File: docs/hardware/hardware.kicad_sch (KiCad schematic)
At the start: 8 parts, among them J1 BASYS_JA, J2 AudioJack2, J6 BASYS_JB, J7 GAMEPAD_1, J8 GAMEPAD_2

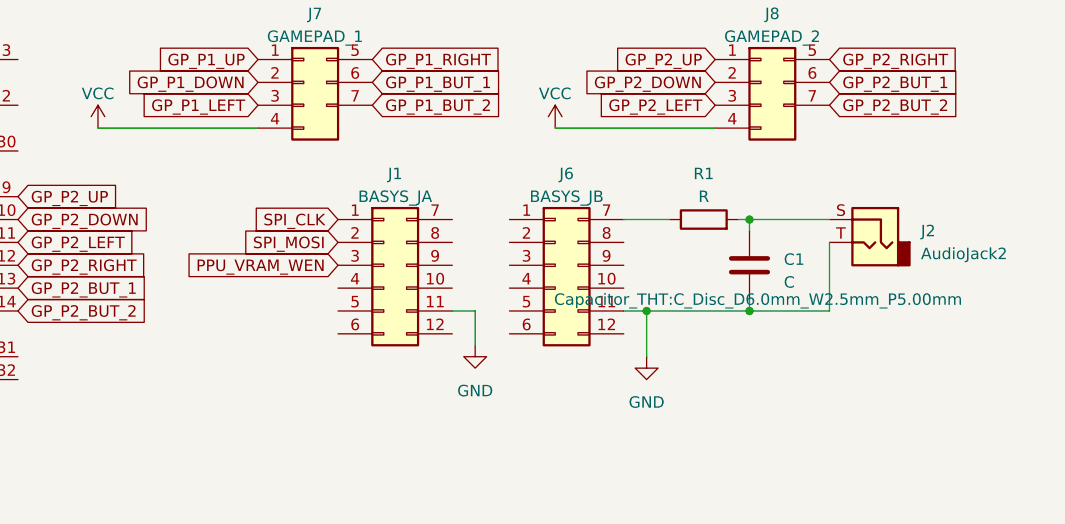
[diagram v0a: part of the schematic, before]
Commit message: WIP ppu testing
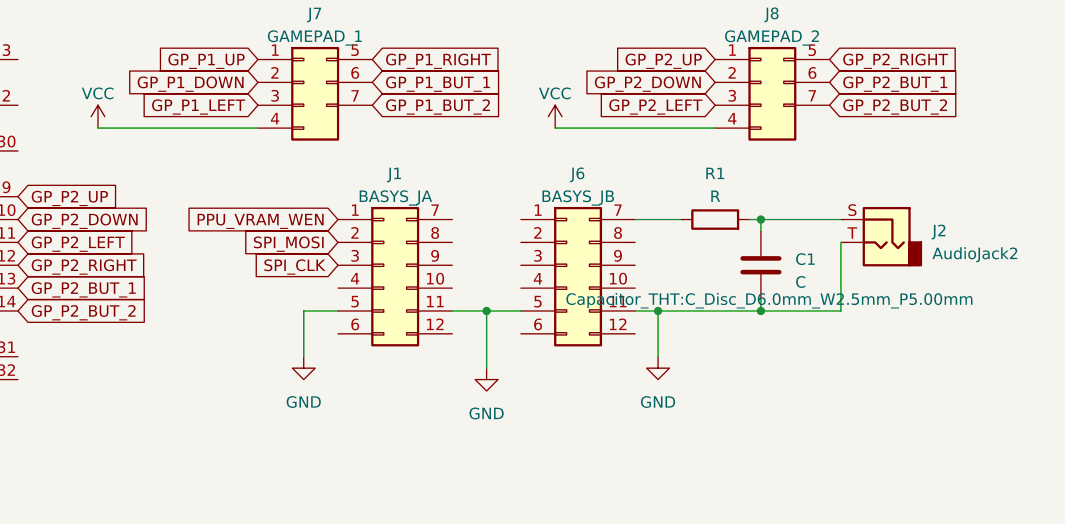
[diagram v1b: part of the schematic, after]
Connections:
- net GND: now also J1.5 (Pin_5), J6.5 (Pin_5)
- net PPU_VRAM_WEN: now also J1.1 (Pin_1); no longer J1.3 (Pin_3)
- net SPI_CLK: now also J1.3 (Pin_3); no longer J1.1 (Pin_1)
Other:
- moved on the sheet: C1, J2, J6, R1

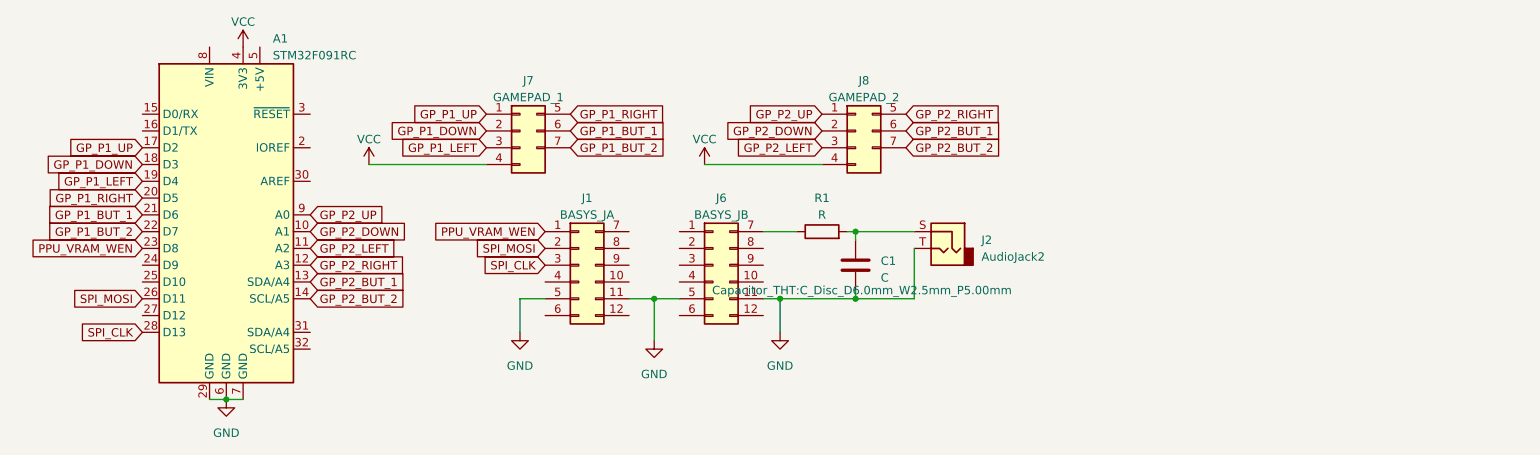
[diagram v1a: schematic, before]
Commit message: finalize hardware
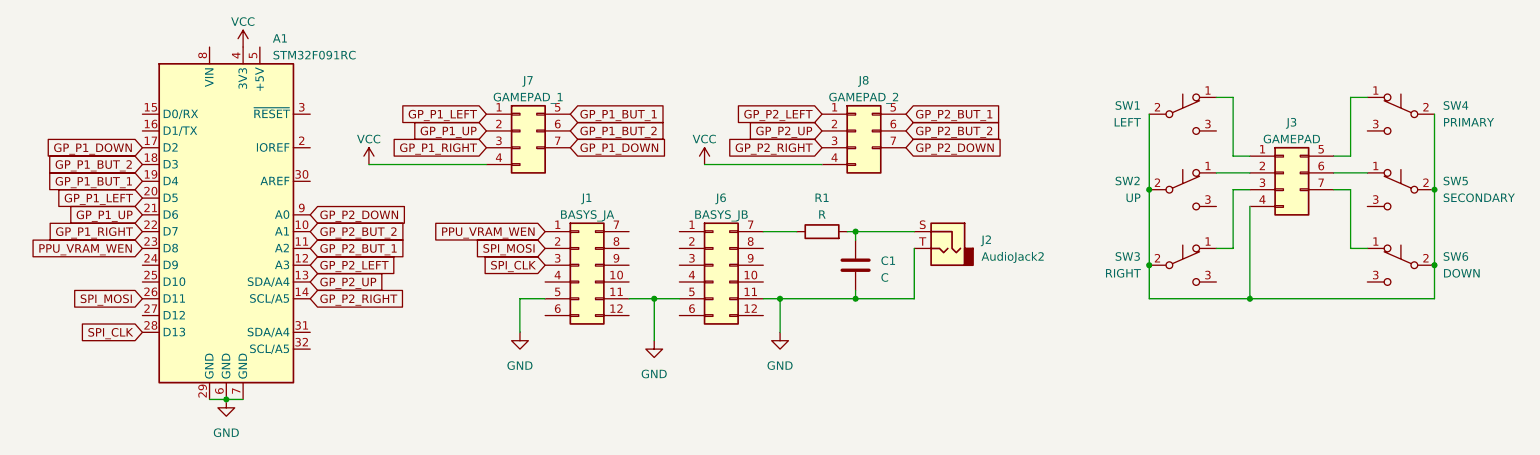
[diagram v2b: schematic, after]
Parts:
- added J3: GAMEPAD, Connector_PinHeader_2.54mm:PinHeader_2x04_P2.54mm_Vertical, symbol Connector_Generic:Conn_02x04_Top_Bottom
- added SW1: LEFT, Button_Switch_THT:SW_PUSH_6mm, symbol Switch:SW_Push_SPDT
- added SW2: UP, Button_Switch_THT:SW_PUSH_6mm, symbol Switch:SW_Push_SPDT
- added SW3: RIGHT, Button_Switch_THT:SW_PUSH_6mm, symbol Switch:SW_Push_SPDT
- added SW4: PRIMARY, Button_Switch_THT:SW_PUSH_6mm, symbol Switch:SW_Push_SPDT
- added SW5: SECONDARY, Button_Switch_THT:SW_PUSH_6mm, symbol Switch:SW_Push_SPDT
- added SW6: DOWN, Button_Switch_THT:SW_PUSH_6mm, symbol Switch:SW_Push_SPDT
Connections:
- net GP_P1_BUT_1: now also A1.19 (D4), J7.5 (RIGHT); no longer A1.21 (D6), J7.6 (PRIMARY)
- net GP_P1_BUT_2: now also A1.18 (D3), J7.6 (PRIMARY); no longer A1.22 (D7), J7.7 (SECONDARY)
- net GP_P1_DOWN: now also A1.17 (D2), J7.7 (SECONDARY); no longer A1.18 (D3), J7.2 (DOWN)
- net GP_P1_LEFT: now also A1.20 (D5), J7.1 (UP); no longer A1.19 (D4), J7.3 (LEFT)
- net GP_P1_RIGHT: now also A1.22 (D7), J7.3 (LEFT); no longer A1.20 (D5), J7.5 (RIGHT)
- net GP_P1_UP: now also A1.21 (D6), J7.2 (DOWN); no longer A1.17 (D2), J7.1 (UP)
- net GP_P2_BUT_1: now also A1.11 (A2), J8.5 (RIGHT); no longer A1.13 (SDA/A4), J8.6 (PRIMARY)
- net GP_P2_BUT_2: now also A1.10 (A1), J8.6 (PRIMARY); no longer A1.14 (SCL/A5), J8.7 (SECONDARY)
- net GP_P2_DOWN: now also A1.9 (A0), J8.7 (SECONDARY); no longer A1.10 (A1), J8.2 (DOWN)
- net GP_P2_LEFT: now also A1.12 (A3), J8.1 (UP); no longer A1.11 (A2), J8.3 (LEFT)
- net GP_P2_RIGHT: now also A1.14 (SCL/A5), J8.3 (LEFT); no longer A1.12 (A3), J8.5 (RIGHT)
- net GP_P2_UP: now also A1.13 (SDA/A4), J8.2 (DOWN); no longer A1.9 (A0), J8.1 (UP)
- new net: J3.5 (RIGHT), SW4.1 (A)
- new net: J3.4 (VCC), SW1.2 (B), SW2.2 (B), SW3.2 (B), SW4.2 (B), SW5.2 (B), SW6.2 (B)
- new net: J3.2 (DOWN), SW2.1 (A)
- new net: J3.1 (UP), SW1.1 (A)
- new net: J3.3 (LEFT), SW3.1 (A)
- new net: J3.6 (PRIMARY), SW5.1 (A)
- new net: J3.7 (SECONDARY), SW6.1 (A)
